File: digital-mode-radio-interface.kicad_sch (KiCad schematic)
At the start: 0 parts

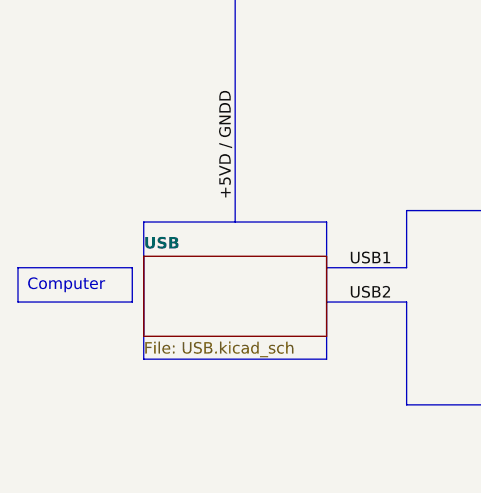
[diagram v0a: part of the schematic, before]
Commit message: kiCAD 9.0
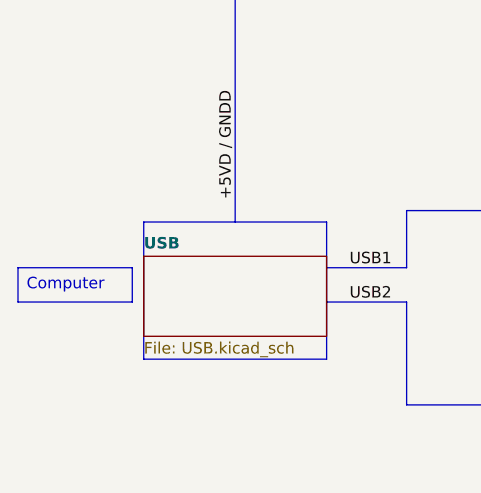
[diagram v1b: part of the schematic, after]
